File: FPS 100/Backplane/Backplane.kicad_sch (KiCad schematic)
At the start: 27 parts

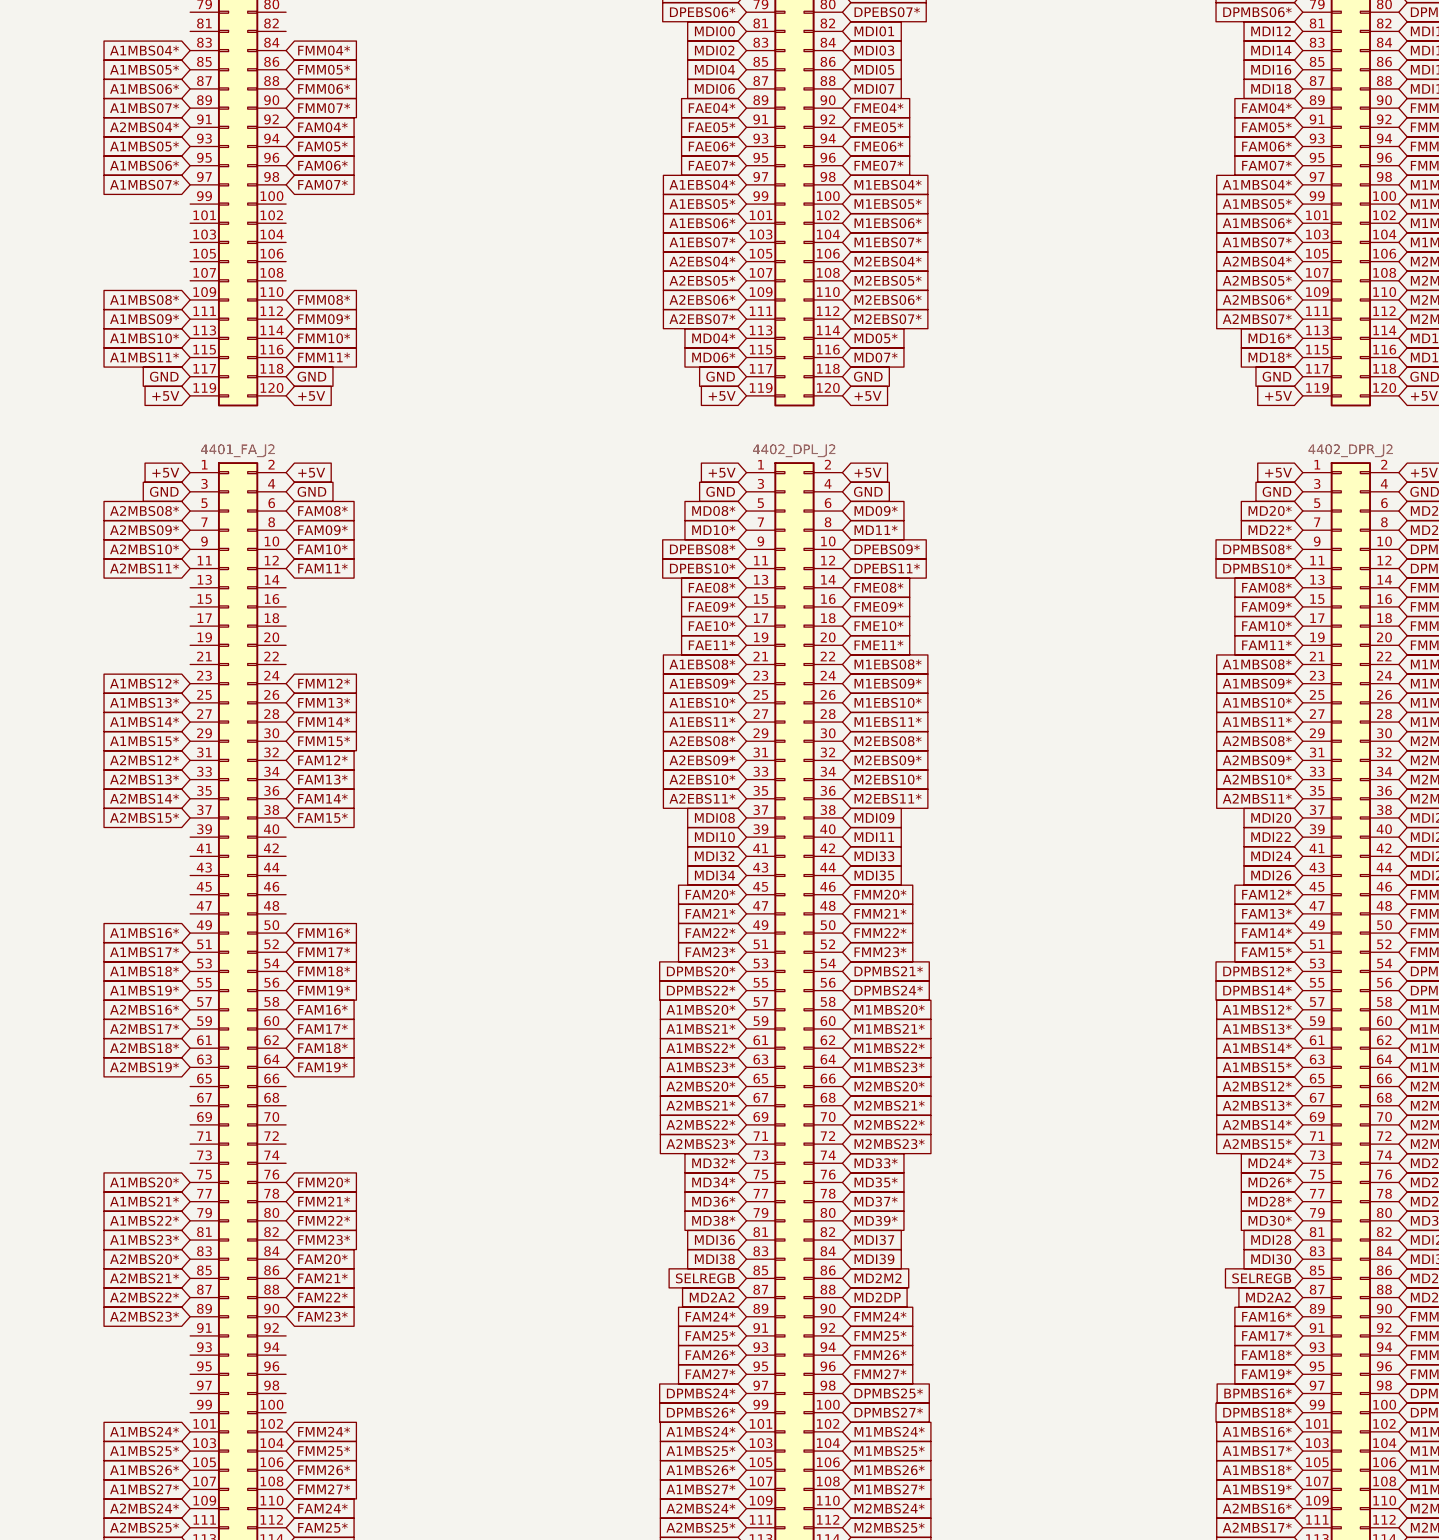
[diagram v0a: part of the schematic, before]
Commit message: 2026/1/6
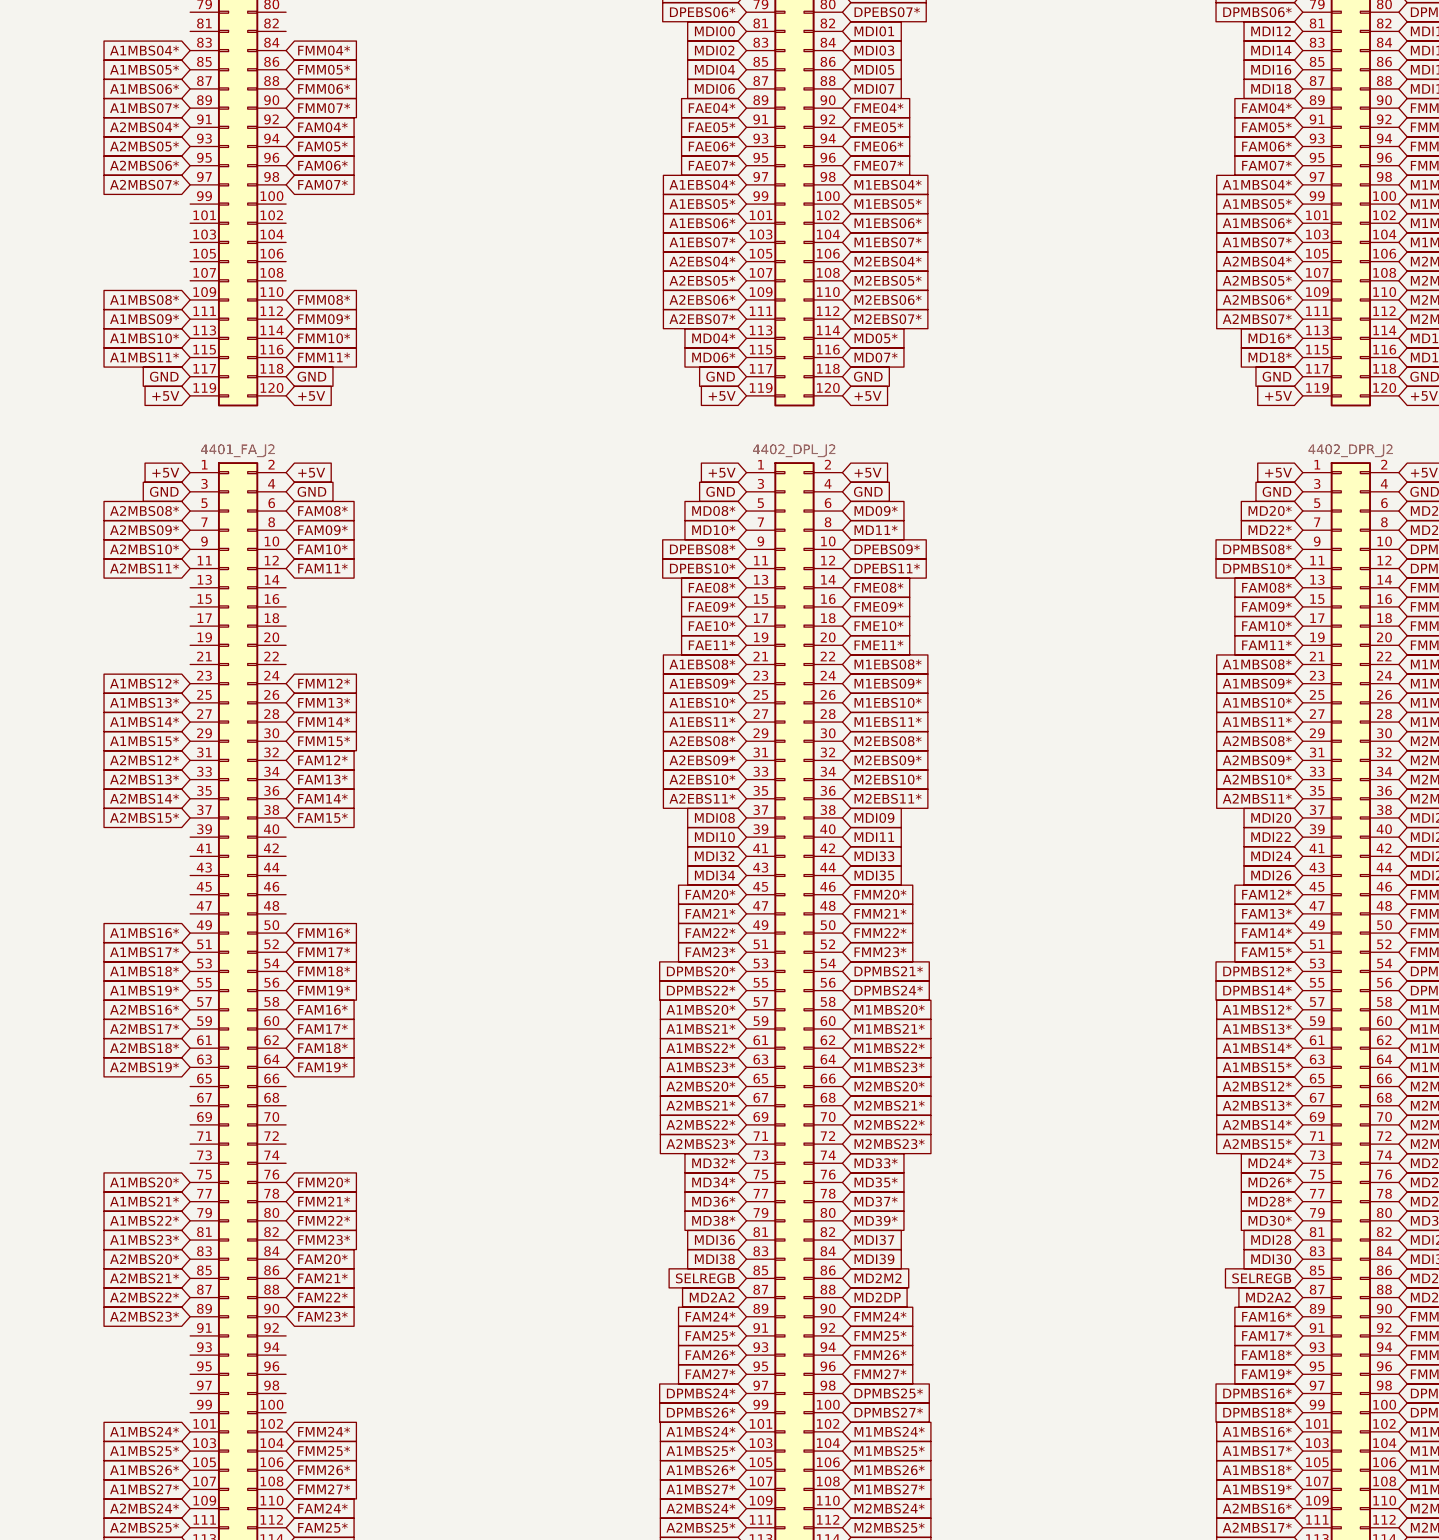
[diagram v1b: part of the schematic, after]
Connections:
- net BPMBS16* is gone; now on net DPMBS16*: 4402_DPR_J2.97
- net A1MBS05*: no longer 4401_FA_J1.93
- net A1MBS06*: no longer 4401_FA_J1.95
- net A1MBS07*: no longer 4401_FA_J1.97
- net A2MBS05*: now also 4401_FA_J1.93
- net A2MBS06*: now also 4401_FA_J1.95
- net A2MBS07*: now also 4401_FA_J1.97
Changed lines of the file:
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@@
 		)
 	)
-	(global_label "A1MBS05*"
+	(global_label "A2MBS05*"
 		(shape input)
 		(at 86.36 179.07 180)
@@
 		)
 	)
-	(global_label "A1MBS07*"
+	(global_label "A2MBS07*"
 		(shape input)
 		(at 86.36 184.15 180)
@@
 		)
 	)
-	(global_label "A1MBS06*"
+	(global_label "A2MBS06*"
 		(shape input)
 		(at 86.36 181.61 180)
@@
 		)
 	)
-	(global_label "BPMBS16*"
+	(global_label "DPMBS16*"
 		(shape input)
 		(at 233.68 344.17 180)
